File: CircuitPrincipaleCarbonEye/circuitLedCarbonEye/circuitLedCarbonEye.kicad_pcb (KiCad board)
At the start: 2 copper layers, 40 x 56 mm, 10 parts, among them J1 4P4C

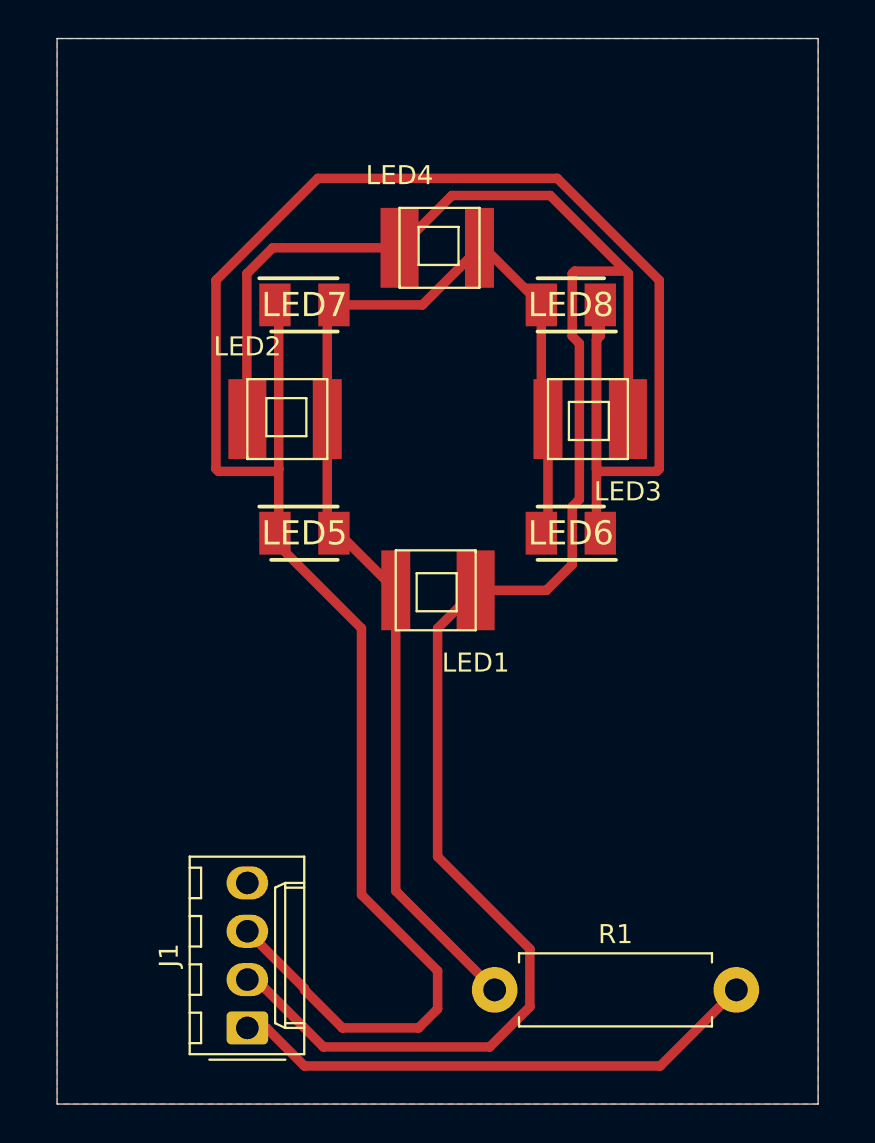
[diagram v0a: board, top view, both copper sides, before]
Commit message: KICAD RoutageCircuit led V1.0
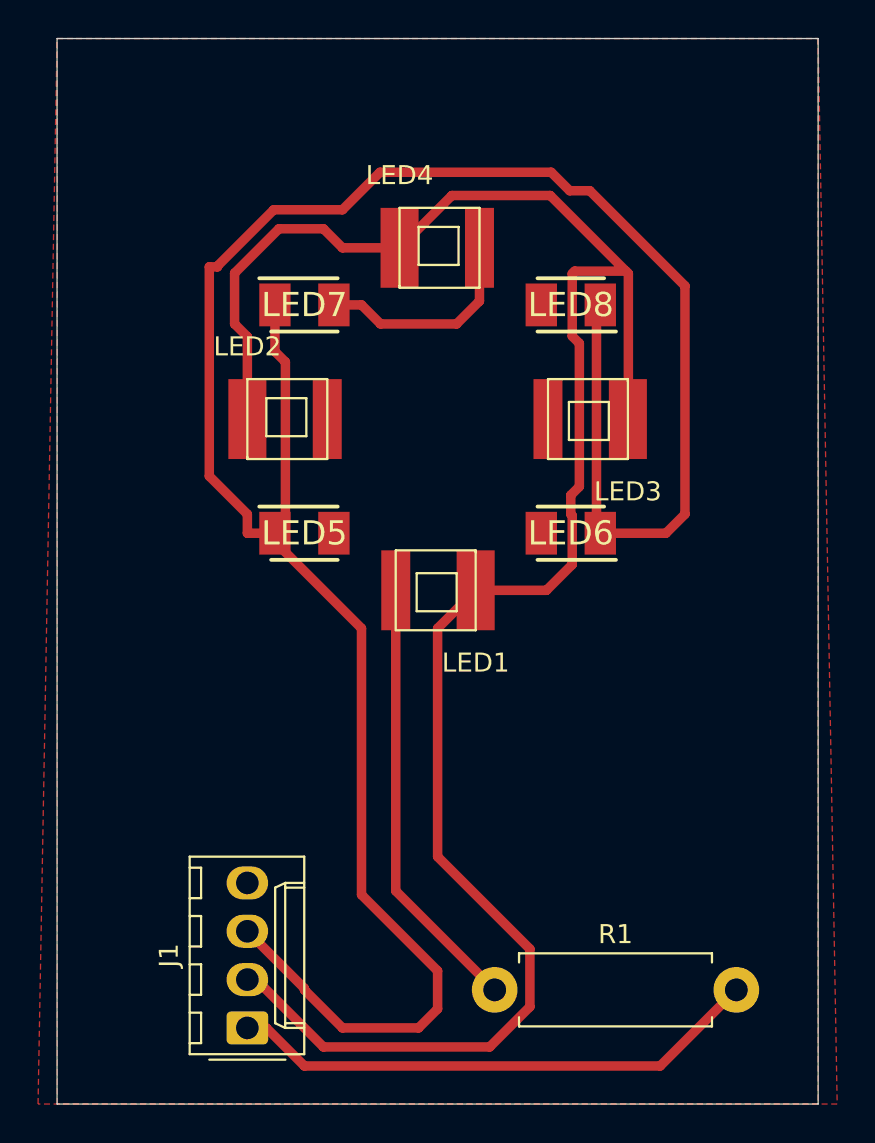
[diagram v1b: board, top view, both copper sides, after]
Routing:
- net Net-(LED1-Pad2): track 65.6 -> 34.5 mm
- net Net-(J1-Pad2): track 105.0 -> 106.8 mm
- added copper zone on F.Cu, net Net-(LED1-Pad2)
